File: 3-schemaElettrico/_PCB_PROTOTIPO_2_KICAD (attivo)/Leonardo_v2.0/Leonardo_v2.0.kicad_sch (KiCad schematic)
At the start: 17 parts, among them J1 Screw_Terminal_01x02, J2 Conn_01x06_Pin, J3 Conn_01x06_Pin, J4 Conn_01x04_Pin, J5 Conn_01x04_Pin, J6 Conn_01x04_Pin, J7 Conn_01x04_Pin, J8 Screw_Terminal_01x02, J9 Screw_Terminal_01x02, Q1 BC817

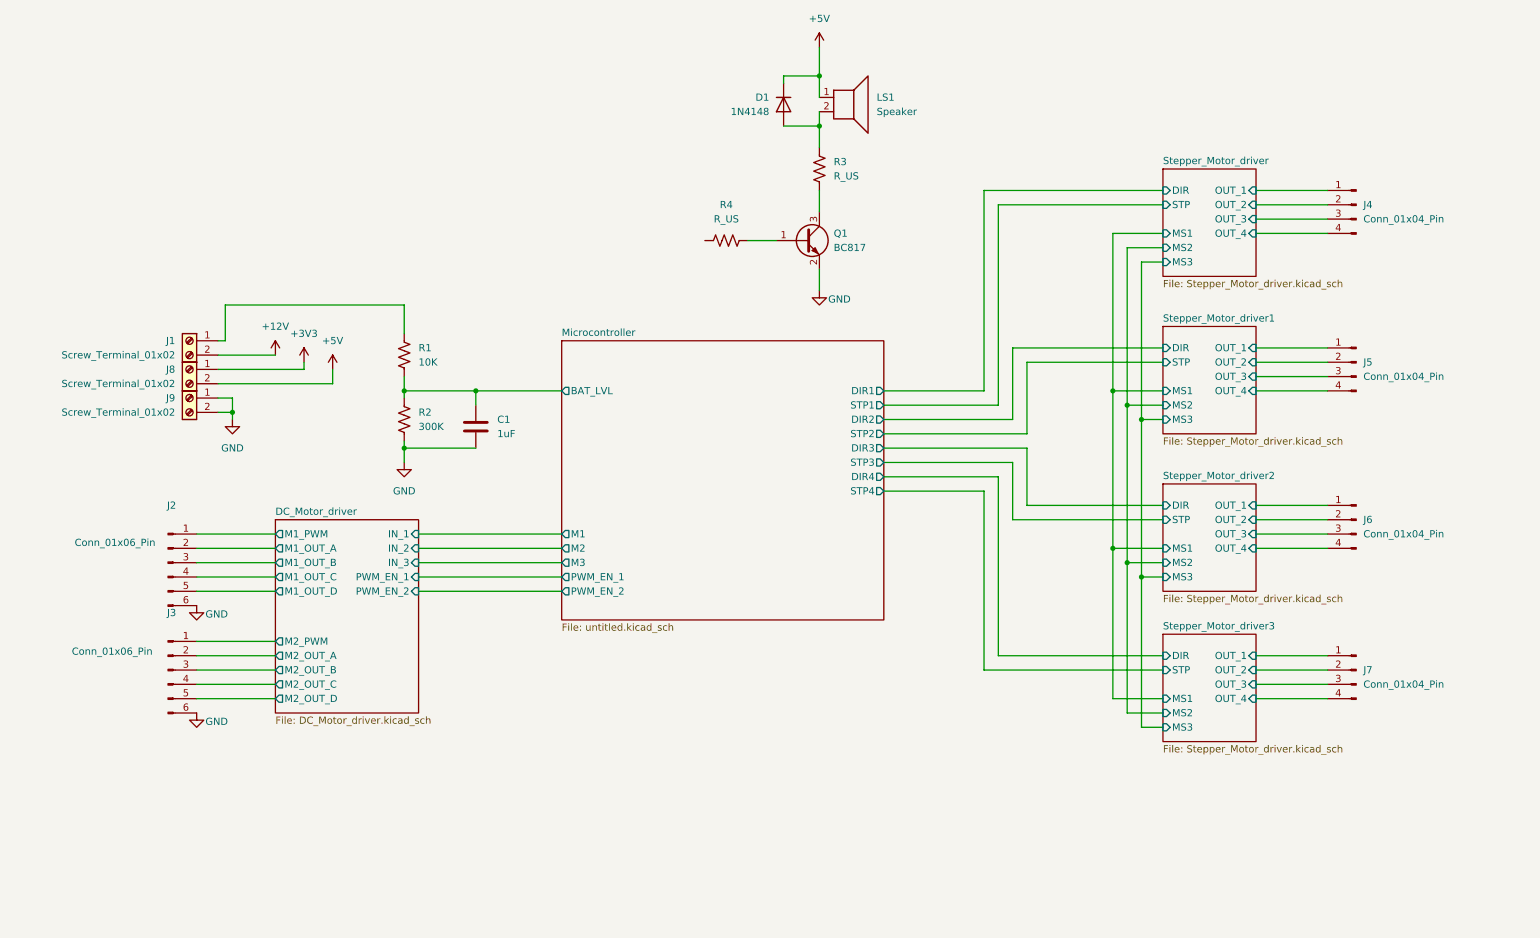
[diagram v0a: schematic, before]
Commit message: ok
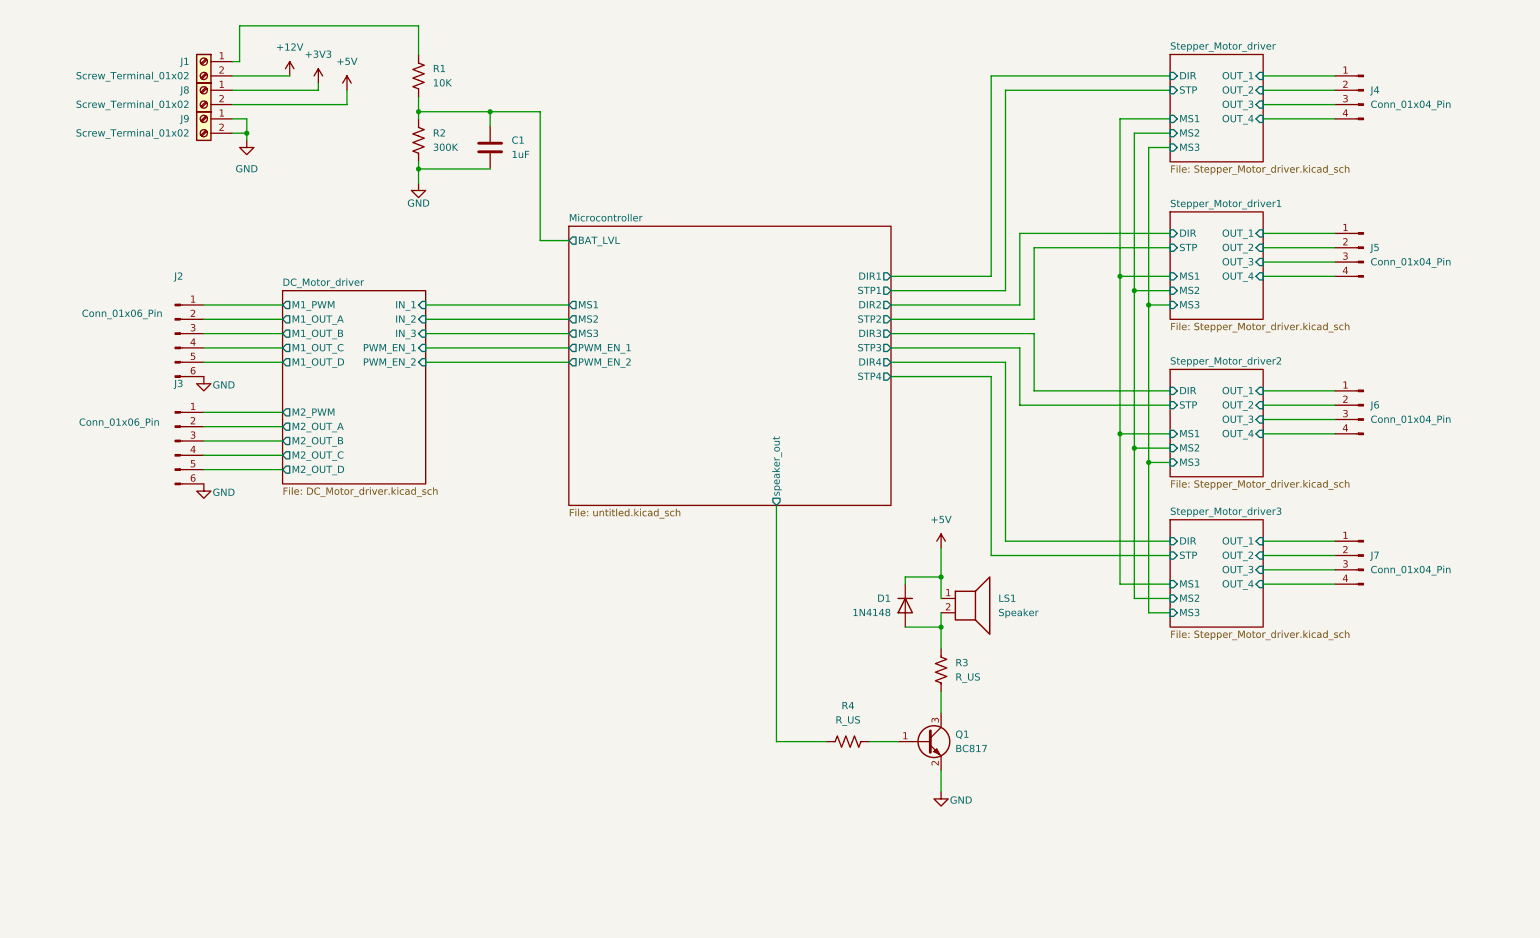
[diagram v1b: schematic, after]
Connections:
- net Microcontroller/speaker_out: now reaches R4.1
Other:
- sheet Microcontroller ports: added MS1, MS2, MS3, speaker_out; removed M1, M2, M3
- moved on the sheet: C1, D1, J1, J2, J3, J4, J5, J6, J7, J8, J9, LS1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

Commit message: semplificato
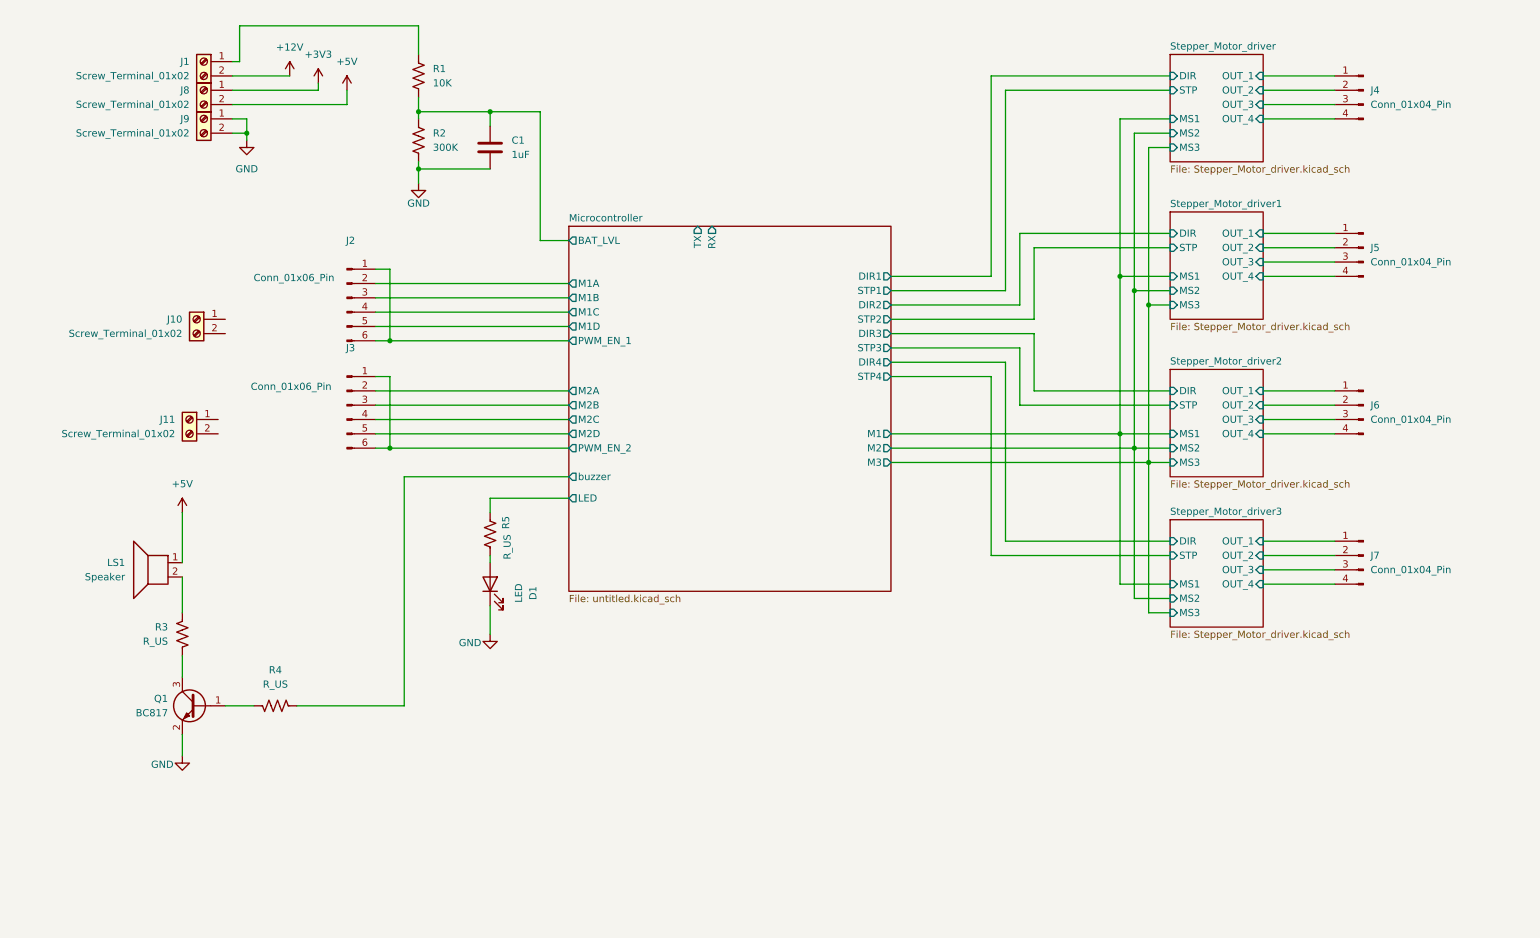
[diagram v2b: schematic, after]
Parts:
- removed D1: 1N4148, Diode_THT:D_DO-35_SOD27_P7.62mm_Horizontal, symbol Diode:1N4148
- added D1: LED, symbol Device:LED
- added J10, J11: Screw_Terminal_01x02, symbol Connector:Screw_Terminal_01x02
- added R5: R_US, symbol Device:R_US
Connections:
- net GND: now also D1.1 (K); no longer J2.6 (Pin_6), J3.6 (Pin_6)
- net DC_Motor_driver/M1_OUT_A renamed Microcontroller/M1A
- net DC_Motor_driver/M1_OUT_B renamed Microcontroller/M1B
- net DC_Motor_driver/M1_OUT_C renamed Microcontroller/M1C
- net DC_Motor_driver/M1_OUT_D renamed Microcontroller/M1D
- net DC_Motor_driver/M1_PWM renamed Microcontroller/PWM_EN_1
- net Microcontroller/PWM_EN_1: now also J2.6 (Pin_6)
- net DC_Motor_driver/M2_OUT_A renamed Microcontroller/M2A
- net DC_Motor_driver/M2_OUT_B renamed Microcontroller/M2B
- net DC_Motor_driver/M2_OUT_C renamed Microcontroller/M2C
- net DC_Motor_driver/M2_OUT_D renamed Microcontroller/M2D
- net DC_Motor_driver/M2_PWM renamed Microcontroller/PWM_EN_2
- net Microcontroller/PWM_EN_2: now also J3.6 (Pin_6)
- net Microcontroller/speaker_out renamed Microcontroller/buzzer
- new net: D1.2 (A), R5.2
- new net Microcontroller/LED: R5.1
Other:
- removed sheet DC_Motor_driver
- sheet Microcontroller ports: added LED, M1, M1A, M1B, M1C, M1D, M2, M2A, M2B, M2C, M2D, M3, RX, TX, buzzer; removed MS1, MS2, MS3, speaker_out
- moved on the sheet: J2, J3, LS1, Q1, R3, R4

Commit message: OK
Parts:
- C1: footprint (none) -> Capacitor_SMD:C_0805_2012Metric_Pad1.18x1.45mm_HandSolder
- D1: footprint (none) -> LED_THT:LED_D3.0mm_FlatTop
- J1, J10, J11, J8, J9: footprint (none) -> TerminalBlock_Phoenix:TerminalBlock_Phoenix_MKDS-1,5-2_1x02_P5.00mm_Horizontal
- J2, J3: footprint (none) -> Connector_PinHeader_2.54mm:PinHeader_1x06_P2.54mm_Vertical
- J4, J5, J6, J7: footprint (none) -> Connector_PinHeader_2.54mm:PinHeader_1x04_P2.54mm_Vertical
- LS1: footprint (none) -> Buzzer_Beeper:Buzzer_TDK_PS1240P02BT_D12.2mm_H6.5mm
- Q1: footprint Package_TO_SOT_SMD:SOT-23 -> Package_TO_SOT_SMD:SOT-23-3
- R1, R2, R3, R4, R5: footprint (none) -> Resistor_SMD:R_0805_2012Metric
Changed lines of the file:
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@@
 			)
 		)
-		(property "Footprint" ""
+		(property "Footprint" "Connector_PinHeader_2.54mm:PinHeader_1x06_P2.54mm_Vertical"
 			(at 73.66 88.9 0)
 			(effects
@@
 			)
 		)
-		(property "Footprint" ""
+		(property "Footprint" "LED_THT:LED_D3.0mm_FlatTop"
 			(at 99.06 120.65 0)
 			(effects
@@
 			)
 		)
-		(property "Footprint" "Package_TO_SOT_SMD:SOT-23"
+		(property "Footprint" "Package_TO_SOT_SMD:SOT-23-3"
 			(at 41.91 144.145 0)
 			(effects
@@
 			)
 		)
-		(property "Footprint" ""
+		(property "Footprint" "Resistor_SMD:R_0805_2012Metric"
 			(at 43.434 129.794 90)
 			(effects
@@
 			)
 		)
-		(property "Footprint" ""
+		(property "Footprint" "Connector_PinHeader_2.54mm:PinHeader_1x04_P2.54mm_Vertical"
 			(at 254 88.9 0)
 			(effects
@@
 			)
 		)
-		(property "Footprint" ""
+		(property "Footprint" "TerminalBlock_Phoenix:TerminalBlock_Phoenix_MKDS-1,5-2_1x02_P5.00mm_Horizontal"
 			(at 48.26 27.94 0)
 			(effects
@@
 			)
 		)
-		(property "Footprint" ""
+		(property "Footprint" "Resistor_SMD:R_0805_2012Metric"
 			(at 60.706 141.224 90)
 			(effects
@@
 			)
 		)
-		(property "Footprint" ""
+		(property "Footprint" "Resistor_SMD:R_0805_2012Metric"
 			(at 87.376 30.734 90)
 			(effects
@@
 			)
 		)
-		(property "Footprint" ""
+		(property "Footprint" "Connector_PinHeader_2.54mm:PinHeader_1x04_P2.54mm_Vertical"
 			(at 254 60.96 0)
 			(effects
@@
 			)
 		)
-		(property "Footprint" ""
+		(property "Footprint" "TerminalBlock_Phoenix:TerminalBlock_Phoenix_MKDS-1,5-2_1x02_P5.00mm_Horizontal"
 			(at 48.26 33.02 0)
 			(effects
@@
 			)
 		)
-		(property "Footprint" ""
+		(property "Footprint" "Resistor_SMD:R_0805_2012Metric"
 			(at 87.376 42.164 90)
 			(effects
@@
 			)
 		)
-		(property "Footprint" ""
+		(property "Footprint" "TerminalBlock_Phoenix:TerminalBlock_Phoenix_MKDS-1,5-2_1x02_P5.00mm_Horizontal"
 			(at 46.99 73.66 0)
 			(effects
@@
 			)
 		)
-		(property "Footprint" ""
+		(property "Footprint" "Connector_PinHeader_2.54mm:PinHeader_1x04_P2.54mm_Vertical"
 			(at 254 33.02 0)
 			(effects
@@
 			)
 		)
-		(property "Footprint" ""
+		(property "Footprint" "TerminalBlock_Phoenix:TerminalBlock_Phoenix_MKDS-1,5-2_1x02_P5.00mm_Horizontal"
 			(at 45.72 91.44 0)
 			(effects
@@
 			)
 		)
-		(property "Footprint" ""
+		(property "Footprint" "Connector_PinHeader_2.54mm:PinHeader_1x04_P2.54mm_Vertical"
 			(at 254 115.57 0)
 			(effects
@@
 			)
 		)
-		(property "Footprint" ""
+		(property "Footprint" "Buzzer_Beeper:Buzzer_TDK_PS1240P02BT_D12.2mm_H6.5mm"
 			(at 39.37 121.92 0)
 			(effects
@@
 			)
 		)
-		(property "Footprint" ""
+		(property "Footprint" "Connector_PinHeader_2.54mm:PinHeader_1x06_P2.54mm_Vertical"
 			(at 73.66 69.85 0)
 			(effects
@@
 			)
 		)
-		(property "Footprint" ""
+		(property "Footprint" "TerminalBlock_Phoenix:TerminalBlock_Phoenix_MKDS-1,5-2_1x02_P5.00mm_Horizontal"
 			(at 48.26 38.1 0)
 			(effects
@@
 			)
 		)
-		(property "Footprint" ""
+		(property "Footprint" "Resistor_SMD:R_0805_2012Metric"
 			(at 100.076 112.014 90)
 			(effects
@@
 			)
 		)
-		(property "Footprint" ""
+		(property "Footprint" "Capacitor_SMD:C_0805_2012Metric_Pad1.18x1.45mm_HandSolder"
 			(at 100.0252 46.99 0)
 			(effects

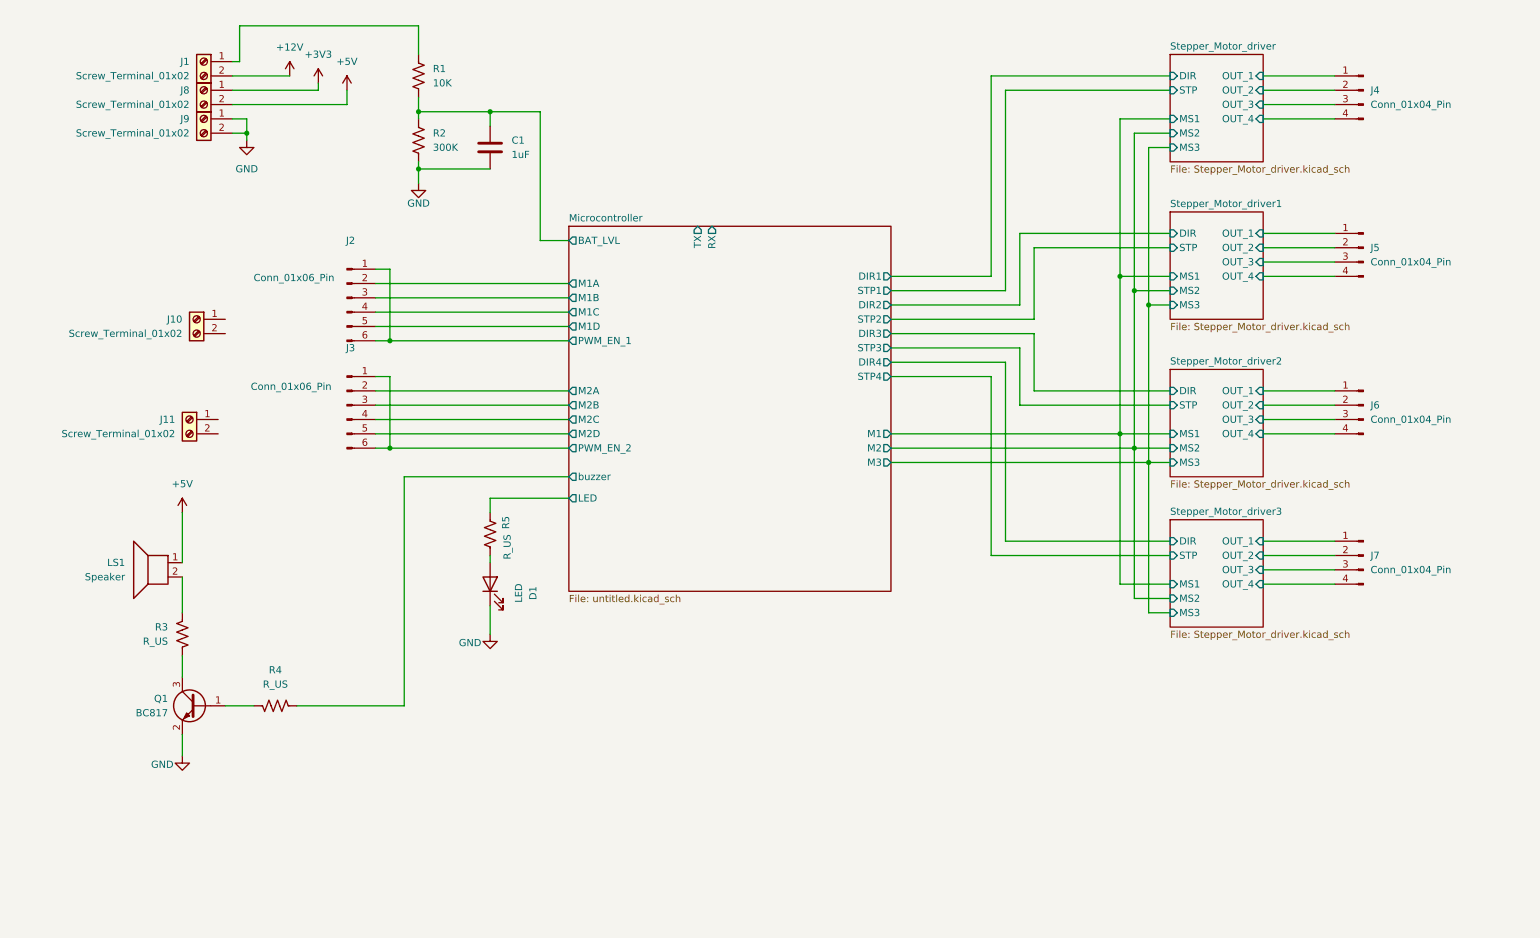
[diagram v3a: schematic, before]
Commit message: ok
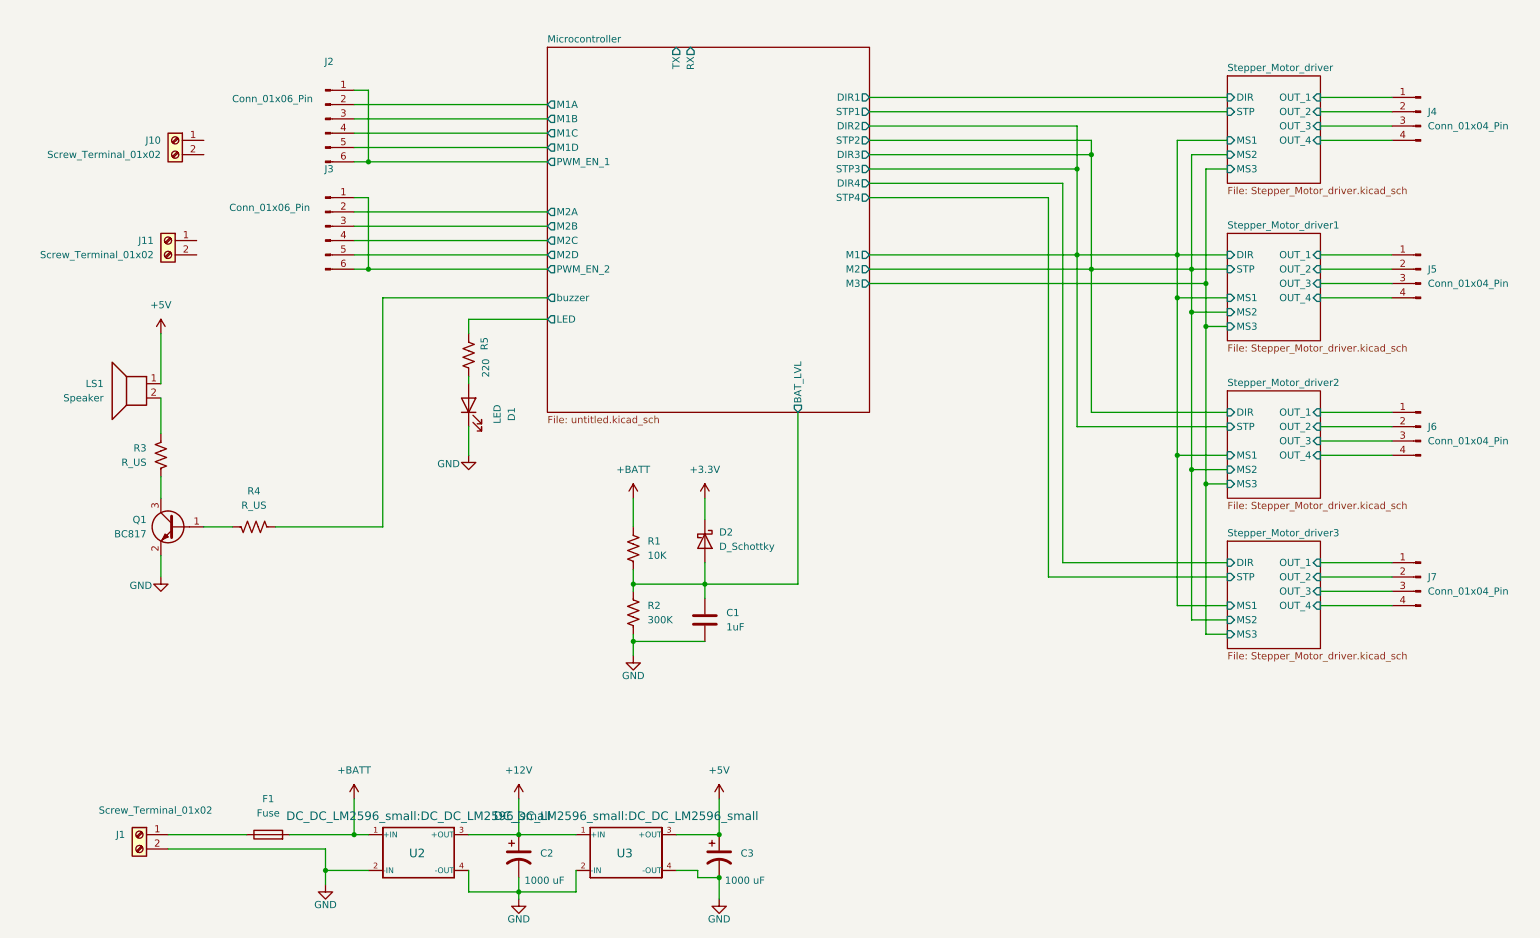
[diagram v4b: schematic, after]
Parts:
- removed J8, J9: Screw_Terminal_01x02, TerminalBlock_Phoenix:TerminalBlock_Phoenix_MKDS-1,5-2_1x02_P5.00mm_Horizontal, symbol Connector:Screw_Terminal_01x02
- added C2, C3: 1000 uF, Capacitor_THT:CP_Radial_D10.0mm_P5.00mm, symbol Device:C_Polarized_US
- added D2: D_Schottky, Diode_THT:D_5KPW_P12.70mm_Horizontal, symbol Device:D_Schottky
- added F1: Fuse, Fuse:Fuse_1812_4532Metric_Pad1.30x3.40mm_HandSolder, symbol Device:Fuse
- added U2, U3: DC_DC_small, DC_DC_LM2596_small:DC_DC_LM2596_small, symbol Custom_dc_dc_small:DC_DC_small
- R5: value R_US -> 220
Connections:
- net +12V: now also C2.1, U2.3 (+OUT), U3.1 (+IN); no longer J1.2 (Pin_2)
- net +5V: now also C3.1, U3.3 (+OUT)
- net GND: now also J1.2 (Pin_2), C2.2, C3.2, U2.2 (-IN), U2.4 (-OUT), U3.2 (-IN), U3.4 (-OUT)
- net Microcontroller/BAT_LVL: now also D2.2 (A)
- net at J1.1 (Pin_1): now also F1.1; no longer R1.1
- new net +3.3V: D2.1 (K)
- new net +BATT: F1.2, R1.1, U2.1 (+IN)
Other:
- moved on the sheet: C1, D1, J1, J10, J11, J2, J3, J4, J5, J6, J7, LS1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
